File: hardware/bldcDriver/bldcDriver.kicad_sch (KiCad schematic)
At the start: 9 parts, among them J1 Conn_01x02, SW1 SW_DPDT_x2, U1 STM32G431CBUx, U2 TPS61088RHLR

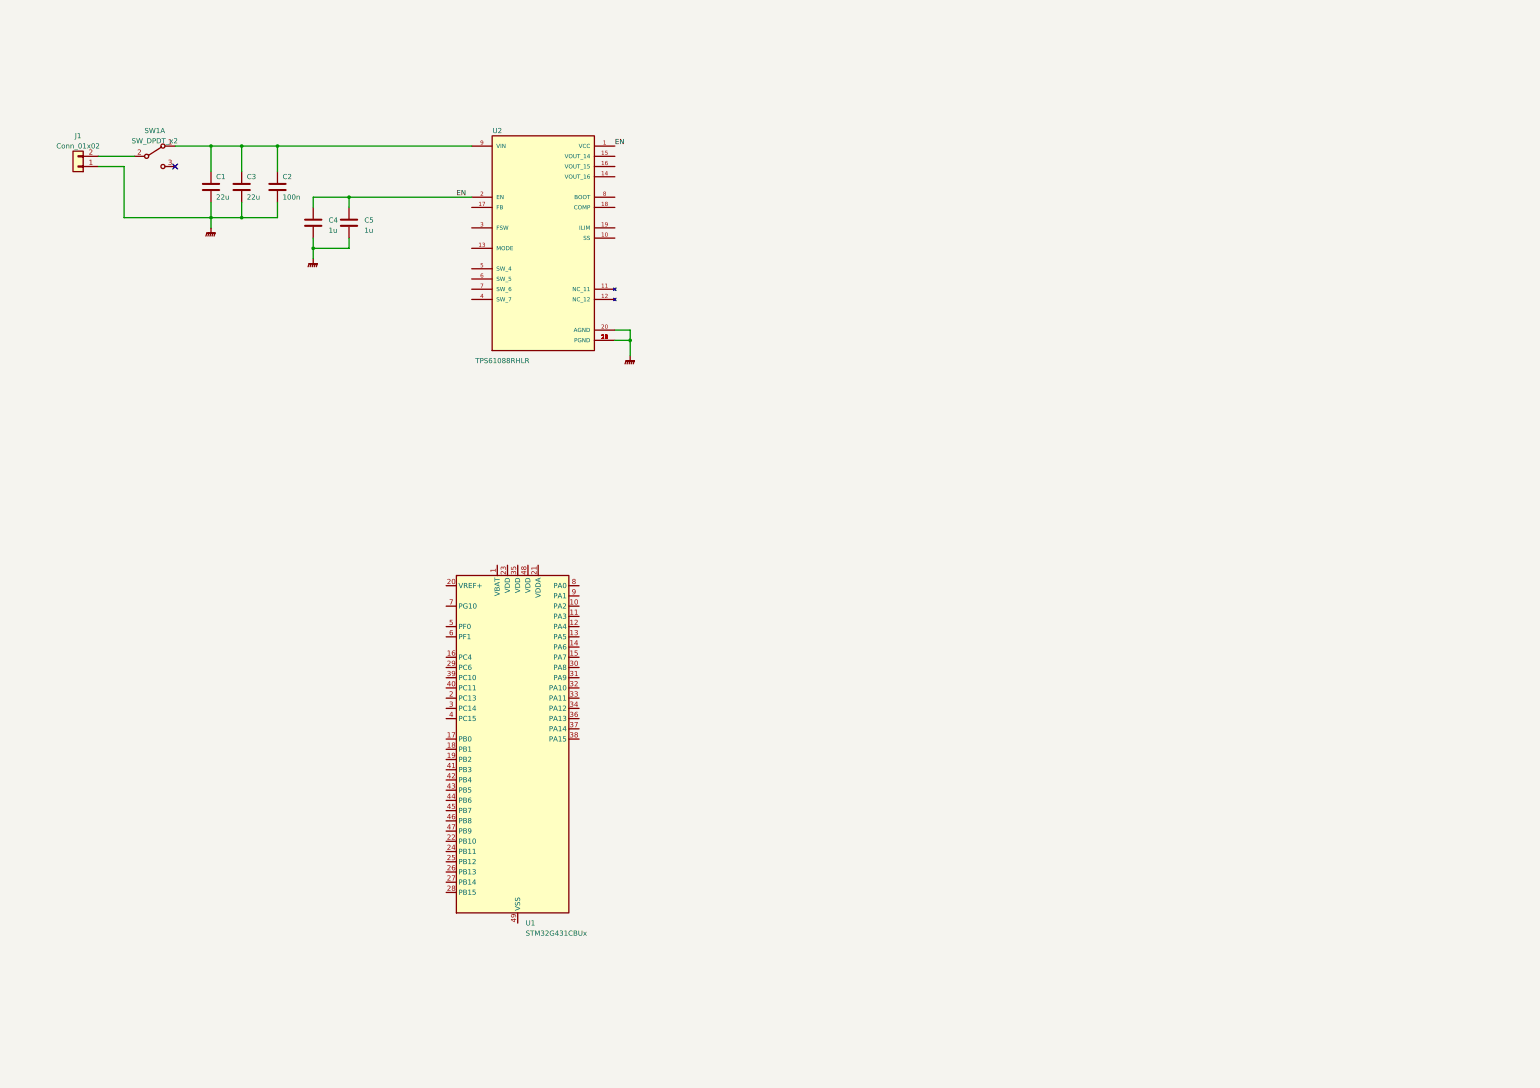
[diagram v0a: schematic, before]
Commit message: bldcDriver sch update
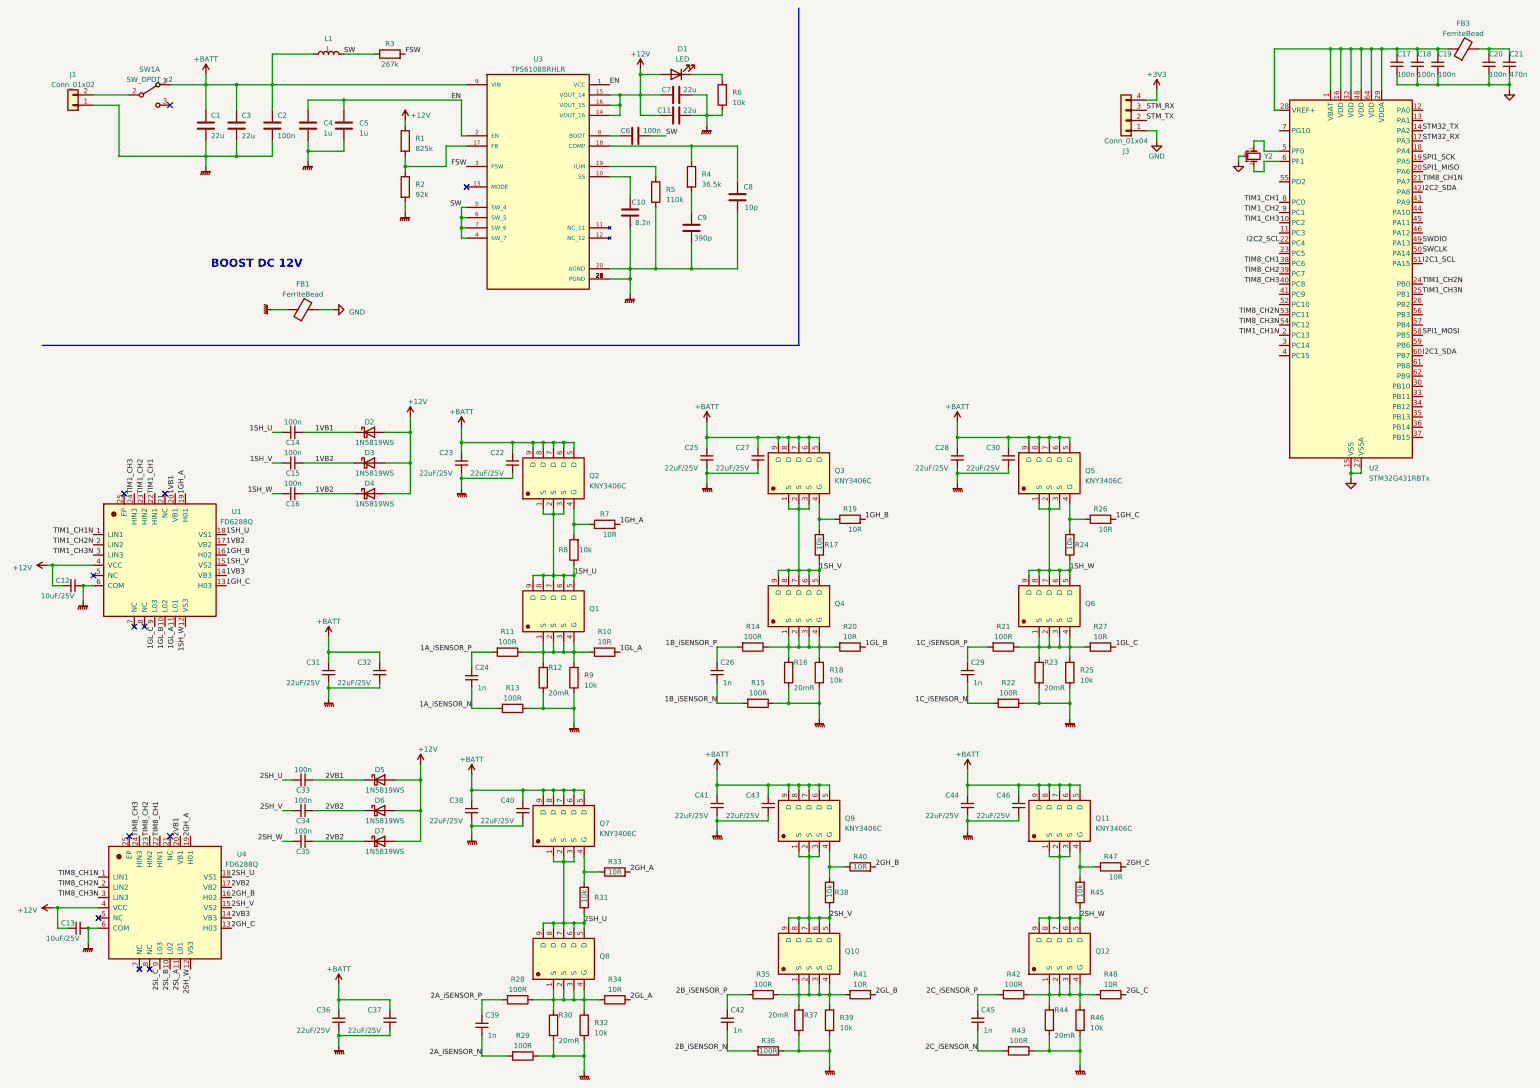
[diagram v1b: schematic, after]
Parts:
- removed U1: STM32G431CBUx, Package_DFN_QFN:QFN-48-1EP_7x7mm_P0.5mm_EP5.6x5.6mm, symbol MCU_ST_STM32G4:STM32G431CBUx
- removed U2: TPS61088RHLR, dp:IC_TPS61088RHLR, symbol dp:TPS61088RHLR
- added C10: 8.2n, symbol Device:C
- added C11, C7: 22u, symbol Device:C
- added C12, C13: 10uF/25V, symbol Device:C_Small
- added C14, C15, C16, C17, C18, C19, C20, C33, C34, C35: 100n, symbol Device:C_Small
- added C21: 470n, symbol Device:C_Small
- added C22, C23, C25, C27, C28, C30, C31, C32, C36, C37, C38, C40, C41, C43, C44, C46: 22uF/25V, symbol Device:C_Small
- added C24, C26, C29, C39, C42, C45: 1n, symbol Device:C_Small
- added C6: 100n, symbol Device:C
- added C8: 10p, symbol Device:C
- added C9: 390p, symbol Device:C
- added D1: LED, symbol Device:LED
- added D2, D3, D4, D5, D6, D7: 1N5819WS, Diode_SMD:D_SOD-323, symbol Diode:1N5819WS
- added FB1, FB3: FerriteBead, symbol Device:FerriteBead
- added J3: Conn_01x04, bat_rf:CONN-SMD_4P-P2.54_XH2.54-4AB_vertical, symbol Connector_Generic:Conn_01x04
- added L1: L, symbol Device:L
- added Q1, Q10, Q11, Q12, Q2, Q3, Q4, Q5, Q6, Q7, Q8, Q9: KNY3406C, kicad_lceda:PDFN-8_L4.9-W5.8-P1.27-LS6.1-BL, symbol bldcDriver:KNY3406C
- added R1: 825k, symbol Device:R
- added R10, R19, R20, R26, R27, R33, R34, R40, R41, R47, R48, R7: 10R, symbol Device:R
- added R11, R13, R14, R15, R21, R22, R28, R29, R35, R36, R42, R43: 100R, symbol Device:R
- added R12, R16, R23, R30, R37, R44: 20mR, symbol Device:R
- added R17, R18, R24, R25, R31, R32, R38, R39, R45, R46, R6, R8, R9: 10k, symbol Device:R
- added R2: 92k, symbol Device:R
- added R3: 267k, symbol Device:R
- added R4: 36.5k, symbol Device:R
- added R5: 110k, symbol Device:R
- added U1, U4: FD6288Q, kicad_lceda:QFN-24_L4.0-W4.0-P0.50-BL-EP2.7, symbol bldcDriver:FD6288Q
- added U2: STM32G431RBTx, Package_QFP:LQFP-64_10x10mm_P0.5mm, symbol MCU_ST_STM32G4:STM32G431RBTx
- added U3: TPS61088RHLR, TPS61088RHLR:IC_TPS61088RHLR, symbol bldcDriver:TPS61088RHLR
- added Y2: Crystal_GND2_Small, symbol Device:Crystal_GND2_Small
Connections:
- net EN: now also U3.1 (VCC), U3.2 (EN)
- net GNDPWR: now also C10.1, C11.2, C12.2, C13.2, C22.2, C23.2, C25.2, C27.2, C28.2, C30.2, C31.2, C32.2, C36.2, C37.2, C38.2, C40.2, C41.2, C43.2, C44.2, C46.2, C7.2, C8.1, C9.1, FB1.1, R12.1, R13.1, R15.1, R16.1, R18.1, R2.2, R22.1, R23.1, R25.1, R29.1, R30.1, R32.1, R36.1, R37.1, R39.1, R43.1, R44.1, R46.1, R5.2, R6.1, R9.1, U1.6 (COM), U3.20 (AGND), U3.21 (PGND), U3.22 (PGND), U3.23 (PGND), U3.24 (PGND), U3.25 (PGND), U3.26 (PGND), U3.27 (PGND), U3.28 (PGND), U3.29 (PGND), U4.6 (COM)
- net +BATT: now reaches C1.1, C2.1, C3.1, SW1.1 (A)
- net +BATT: now also C22.1, C23.1, C25.1, C27.1, C28.1, C30.1, C31.1, C32.1, C36.1, C37.1, C38.1, C40.1, C41.1, C43.1, C44.1, C46.1, L1.1, Q11.5 (D), Q11.6 (D), Q11.7 (D), Q11.8 (D), Q11.9 (D), Q2.5 (D), Q2.6 (D), Q2.7 (D), Q2.8 (D), Q2.9 (D), Q3.5 (D), Q3.6 (D), Q3.7 (D), Q3.8 (D), Q3.9 (D), Q5.5 (D), Q5.6 (D), Q5.7 (D), Q5.8 (D), Q5.9 (D), Q7.5 (D), Q7.6 (D), Q7.7 (D), Q7.8 (D), Q7.9 (D), Q9.5 (D), Q9.6 (D), Q9.7 (D), Q9.8 (D), Q9.9 (D), U3.9 (VIN)
- new net: C6.1, U3.8 (BOOT)
- new net: Q10.1 (S), Q10.2 (S), Q10.3 (S), Q10.4 (G), R35.1, R37.2, R39.2, R41.2
- new net: Q3.4 (G), R17.2, R19.1
- new net: Q2.4 (G), R7.1, R8.2
- new net: Q7.4 (G), R31.2, R33.1
- new net: Q12.1 (S), Q12.2 (S), Q12.3 (S), Q12.4 (G), R42.1, R44.2, R46.2, R48.2
- new net: Q9.4 (G), R38.2, R40.1
- new net: Q4.1 (S), Q4.2 (S), Q4.3 (S), Q4.4 (G), R14.1, R16.2, R18.2, R20.2
- new net: Q8.1 (S), Q8.2 (S), Q8.3 (S), Q8.4 (G), R28.1, R30.2, R32.2, R34.2
- new net: U2.5 (PF0), Y2.1
- new net: U2.6 (PF1), Y2.3
- new net: Q1.1 (S), Q1.2 (S), Q1.3 (S), Q1.4 (G), R10.2, R11.1, R12.2, R9.2
- new net: Q5.4 (G), R24.2, R26.1
- new net: C17.1, C18.1, C19.1, FB3.1, U2.1 (VBAT), U2.16 (VDD), U2.28 (VREF+), U2.29 (VDDA), U2.32 (VDD), U2.48 (VDD), U2.64 (VDD)
- new net: C20.1, C21.1, FB3.2
- new net: Q11.4 (G), R45.2, R47.1
- new net: C10.2, U3.10 (SS)
- new net: Q6.1 (S), Q6.2 (S), Q6.3 (S), Q6.4 (G), R21.1, R23.2, R25.2, R27.2
- new net: R1.2, R2.1, U3.17 (FB)
- new net: D1.1 (K), R6.2
- new net: R5.1, U3.19 (ILIM)
- new net: C8.2, R4.1, U3.18 (COMP)
- new net: C9.2, R4.2
- new net +12V: C11.1, C12.1, C13.1, C7.1, D1.2 (A), D2.2 (A), D3.2 (A), D4.2 (A), D5.2 (A), D6.2 (A), D7.2 (A), R1.1, U1.4 (VCC), U3.14 (VOUT_16), U3.15 (VOUT_14), U3.16 (VOUT_15), U4.4 (VCC)
- new net +3V3: J3.4 (Pin_4)
- new net 1A_iSENSOR_N: C24.1, R13.2
- new net 1A_iSENSOR_P: C24.2, R11.2
- new net 1B_iSENSOR_N: C26.1, R15.2
- new net 1B_iSENSOR_P: C26.2, R14.2
- new net 1C_iSENSOR_N: C29.1, R22.2
- new net 1C_iSENSOR_P: C29.2, R21.2
- new net 1GH_A: R7.2, U1.19 (H01)
- new net 1GH_B: R19.2, U1.16 (H02)
- new net 1GH_C: R26.2, U1.13 (H03)
- new net 1GL_A: R10.1, U1.11 (L01)
- new net 1GL_B: R20.1, U1.10 (L02)
- new net 1GL_C: R27.1, U1.9 (L03)
- new net 1SH_U: C14.2, Q1.5 (D), Q1.6 (D), Q1.7 (D), Q1.8 (D), Q1.9 (D), Q2.1 (S), Q2.2 (S), Q2.3 (S), R8.1, U1.18 (VS1)
- new net 1SH_V: C15.2, Q3.1 (S), Q3.2 (S), Q3.3 (S), Q4.5 (D), Q4.6 (D), Q4.7 (D), Q4.8 (D), Q4.9 (D), R17.1, U1.15 (VS2)
- new net 1SH_W: C16.2, Q5.1 (S), Q5.2 (S), Q5.3 (S), Q6.5 (D), Q6.6 (D), Q6.7 (D), Q6.8 (D), Q6.9 (D), R24.1, U1.12 (VS3)
- new net 1VB1: C14.1, D2.1 (K), U1.20 (VB1)
- new net 1VB2: C15.1, C16.1, D3.1 (K), D4.1 (K), U1.17 (VB2)
- new net 1VB3: U1.14 (VB3)
- new net 2A_iSENSOR_N: C39.1, R29.2
- new net 2A_iSENSOR_P: C39.2, R28.2
- new net 2B_iSENSOR_N: C42.1, R36.2
- new net 2B_iSENSOR_P: C42.2, R35.2
- new net 2C_iSENSOR_N: C45.1, R43.2
- new net 2C_iSENSOR_P: C45.2, R42.2
- new net 2GH_A: R33.2, U4.19 (H01)
- new net 2GH_B: R40.2, U4.16 (H02)
- new net 2GH_C: R47.2, U4.13 (H03)
- new net 2GL_A: R34.1
- new net 2GL_B: R41.1
- new net 2GL_C: R48.1
- new net 2SH_U: C33.2, Q7.1 (S), Q7.2 (S), Q7.3 (S), Q8.5 (D), Q8.6 (D), Q8.7 (D), Q8.8 (D), Q8.9 (D), R31.1, U4.18 (VS1)
- new net 2SH_V: C34.2, Q10.5 (D), Q10.6 (D), Q10.7 (D), Q10.8 (D), Q10.9 (D), Q9.1 (S), Q9.2 (S), Q9.3 (S), R38.1, U4.15 (VS2)
- new net 2SH_W: C35.2, Q11.1 (S), Q11.2 (S), Q11.3 (S), Q12.5 (D), Q12.6 (D), Q12.7 (D), Q12.8 (D), Q12.9 (D), R45.1, U4.12 (VS3)
- new net 2SL_A: U4.11 (L01)
- new net 2SL_B: U4.10 (L02)
- new net 2SL_C: U4.9 (L03)
- new net 2VB1: C33.1, D5.1 (K), U4.20 (VB1)
- new net 2VB2: C34.1, C35.1, D6.1 (K), D7.1 (K), U4.17 (VB2)
- new net 2VB3: U4.14 (VB3)
- new net FSW: R3.2, U3.3 (FSW)
- new net GND: C17.2, C18.2, C19.2, C20.2, C21.2, FB1.2, J3.1 (Pin_1), U2.15 (VSS), U2.27 (VSSA), U2.31 (VSS), U2.47 (VSS), U2.63 (VSS), Y2.2
- new net I2C1_SCL: U2.51 (PA15)
- new net I2C1_SDA: U2.60 (PB7)
- new net I2C2_SCL: U2.22 (PC4)
- new net I2C2_SDA: U2.42 (PA8)
- new net SPI1_MISO: U2.20 (PA6)
- new net SPI1_MOSI: U2.58 (PB5)
- new net SPI1_SCK: U2.19 (PA5)
- new net STM32_RX: U2.17 (PA3)
- new net STM32_TX: U2.14 (PA2)
- new net STM_RX: J3.3 (Pin_3)
- new net STM_TX: J3.2 (Pin_2)
- new net SW: C6.2, L1.2, R3.1, U3.4 (SW_7), U3.5 (SW_4), U3.6 (SW_5), U3.7 (SW_6)
- new net SWCLK: U2.50 (PA14)
- new net SWDIO: U2.49 (PA13)
- new net TIM1_CH1: U1.22 (HIN1), U2.8 (PC0)
- new net TIM1_CH1N: U1.1 (LIN1), U2.2 (PC13)
- new net TIM1_CH2: U1.23 (HIN2), U2.9 (PC1)
- new net TIM1_CH2N: U1.2 (LIN2), U2.24 (PB0)
- new net TIM1_CH3: U1.24 (HIN3), U2.10 (PC2)
- new net TIM1_CH3N: U1.3 (LIN3), U2.25 (PB1)
- new net TIM8_CH1: U2.38 (PC6), U4.22 (HIN1)
- new net TIM8_CH1N: U2.21 (PA7), U4.1 (LIN1)
- new net TIM8_CH2: U2.39 (PC7), U4.23 (HIN2)
- new net TIM8_CH2N: U2.53 (PC11), U4.2 (LIN2)
- new net TIM8_CH3: U2.40 (PC8), U4.24 (HIN3)
- new net TIM8_CH3N: U2.54 (PC12), U4.3 (LIN3)
- no-connect marks 1 -> 12
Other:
- note added: "BOOST DC 12V"
- moved on the sheet: C1, C2, C3, C4, C5, J1, SW1A
